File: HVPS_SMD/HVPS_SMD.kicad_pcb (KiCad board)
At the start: 2 copper layers, 30 x 20 mm, 25 parts, among them J1 CONN_01X02, J2 CONN_01X02, J3 CONN_01X02, Q1 AO4294, T1 MagTop-HVSMPS, U1 LM3478SOIC8

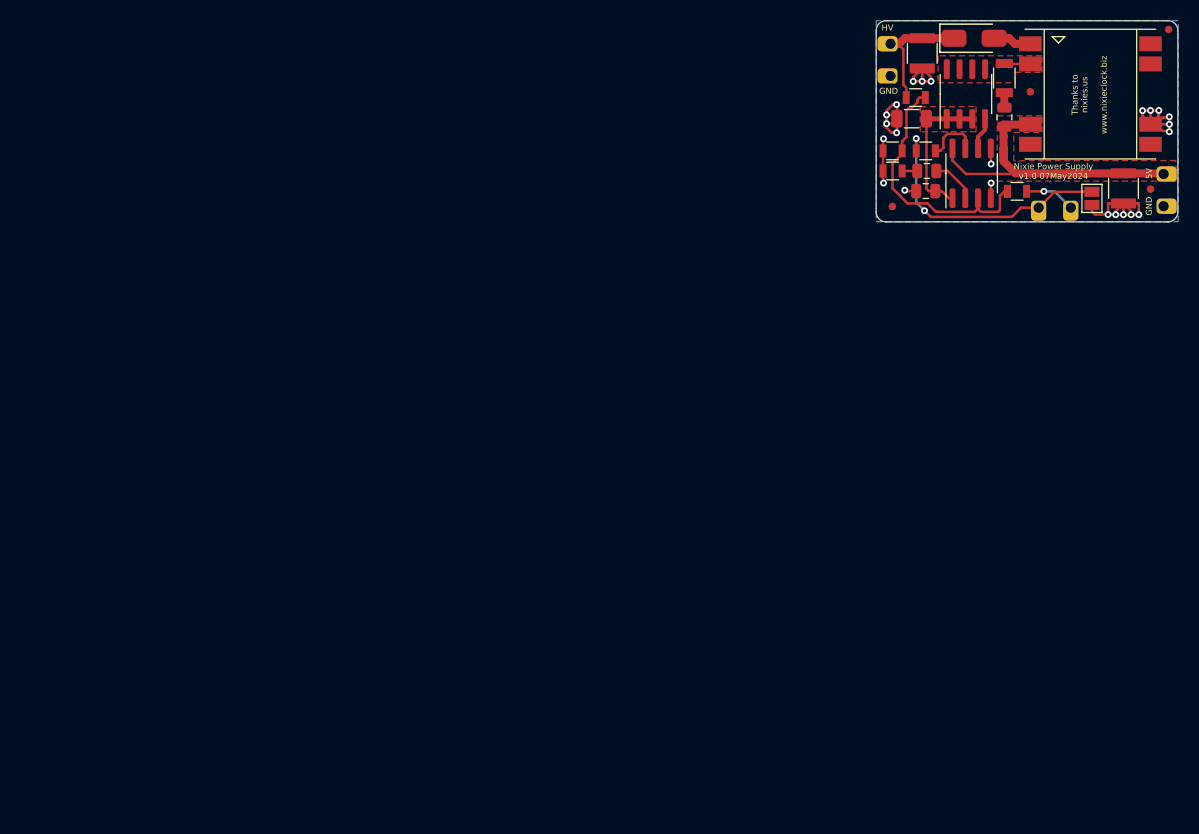
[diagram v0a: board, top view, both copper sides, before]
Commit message: Correct LCSC Part #
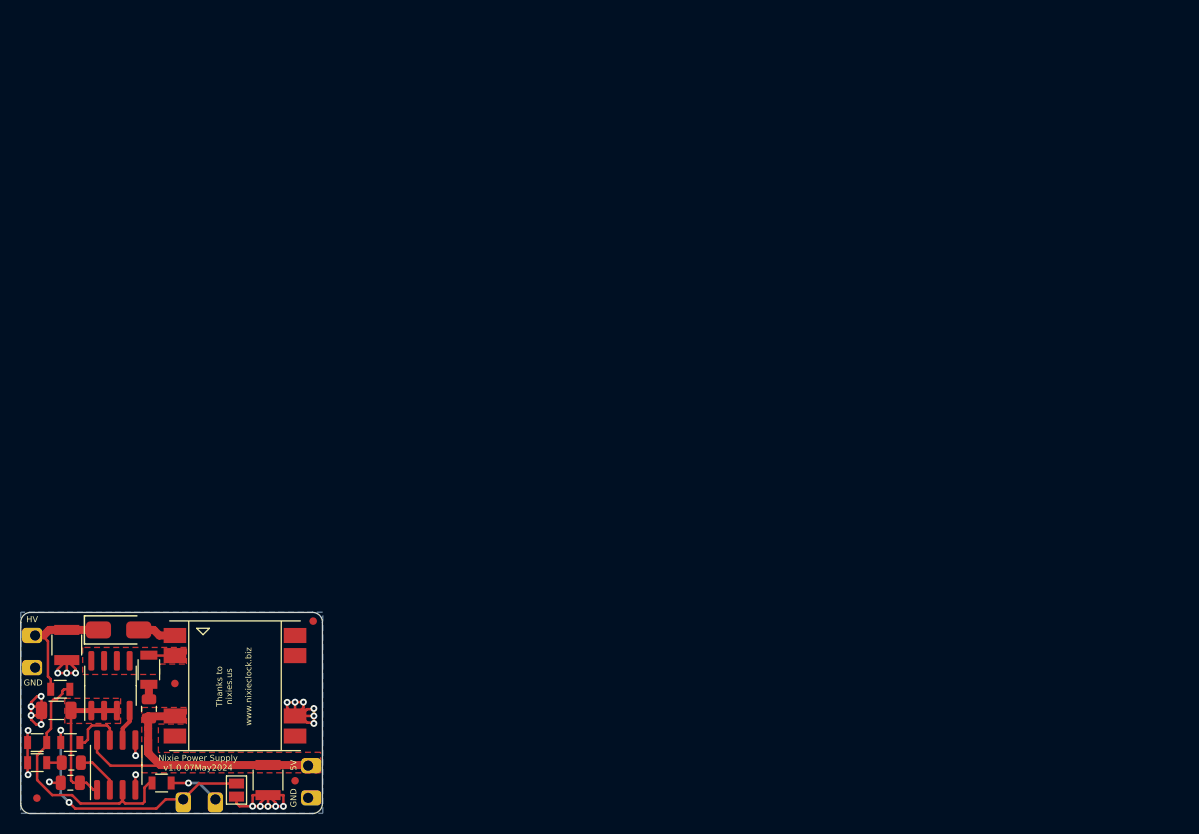
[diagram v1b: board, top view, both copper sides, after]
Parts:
- moved FID3 103.4 mm to (115.3, 127.1)
- moved FID4 103.4 mm to (101.6, 138.5)
- moved Rs1 103.4 mm to (112.7, 125.7)
- moved C2 103.4 mm to (104.9, 136.9)
- moved C3 103.4 mm to (104.6, 123.2)
- moved Cc1 103.4 mm to (105.0, 134.9)
- moved Cs1 103.4 mm to (112.8, 129.6)
- moved D1 103.4 mm to (109.7, 121.7)
- moved FID1 103.4 mm to (127.3, 136.7)
- moved FID2 103.4 mm to (129.1, 120.9)
- moved G*** 103.4 mm to (115.4, 127.9)
- moved J1 103.4 mm to (128.6, 136.8)
- moved J2 103.4 mm to (101.4, 123.9)
- moved J3 103.4 mm to (117.8, 138.6)
- moved JP1 103.4 mm to (121.5, 137.7)
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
